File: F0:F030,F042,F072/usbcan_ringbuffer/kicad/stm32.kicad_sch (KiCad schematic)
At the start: 54 parts, among them J1 Screw_Terminal_01x03, J10 SDA, J11 PB0, J12 PB1, J13 PB4, J14 PB5, J15 PB2, J16 PB3, J17 GND, J18 GND, J19 +3.3V, J2 SCK, J20 +5V, J21 PA0, J22 PA1, J23 PA2, J24 PA3, J25 PB10, J26 PB11, J3 SWDetc, J4 USB_B, J5 MISO, J6 MOSI, J7 TX, J8 RX, J9 SCL, P1 Hole, P2 Hole, P3 Hole, P4 Hole, Q1 B0505S, SW1 SW_DIP_x01, U1 LM1117-3.3, U2 USBLC6-2SC6, U3 STM32F072C8Tx, U4 ISO1050DUB

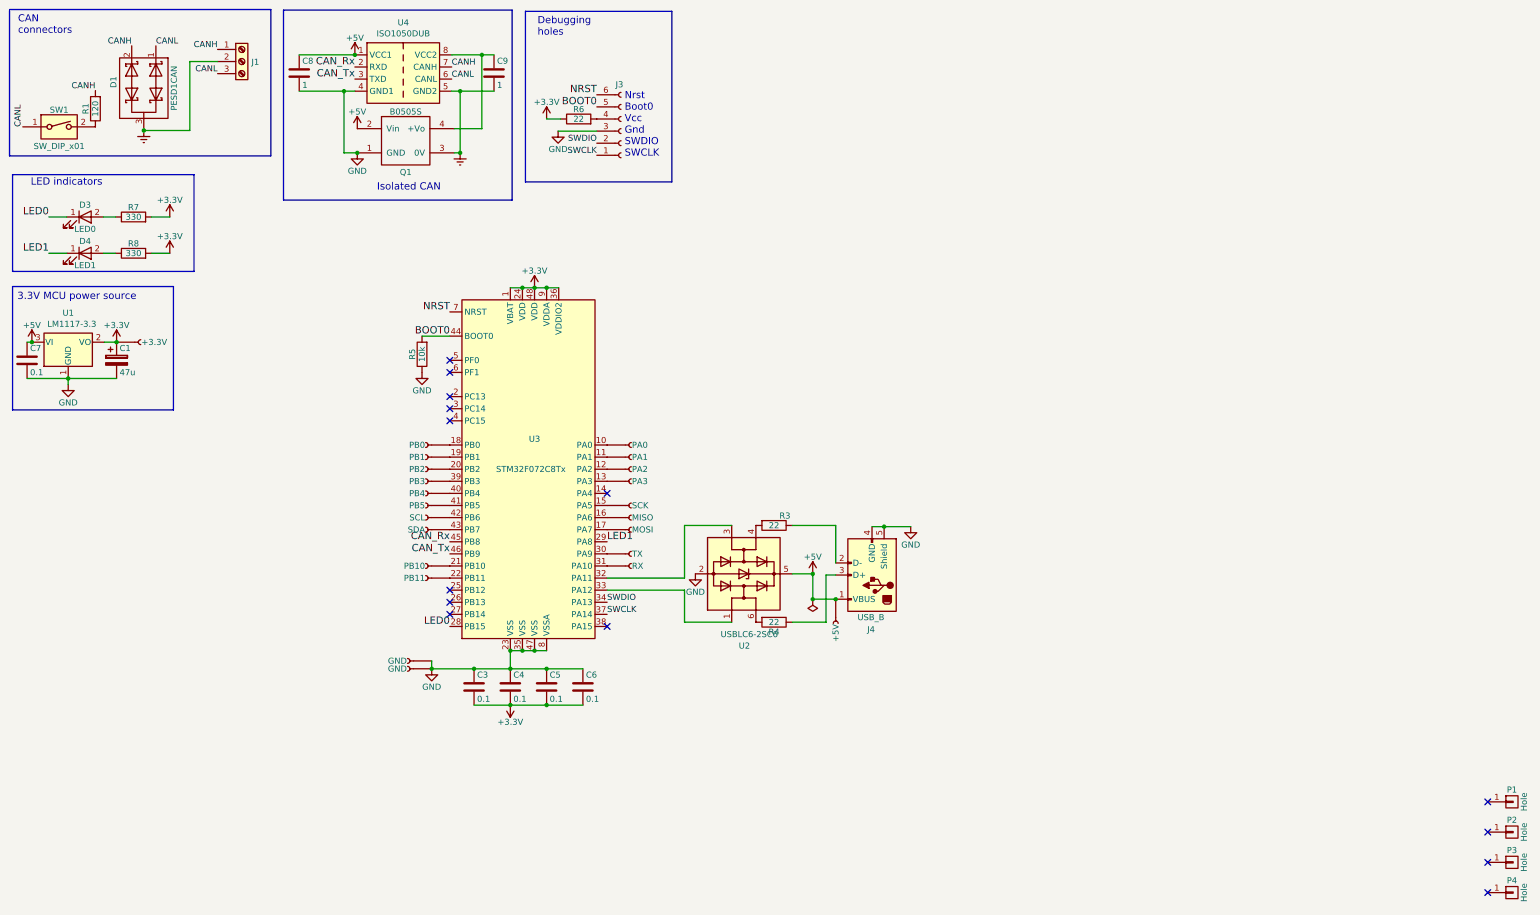
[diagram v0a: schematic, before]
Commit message: save under new kicad
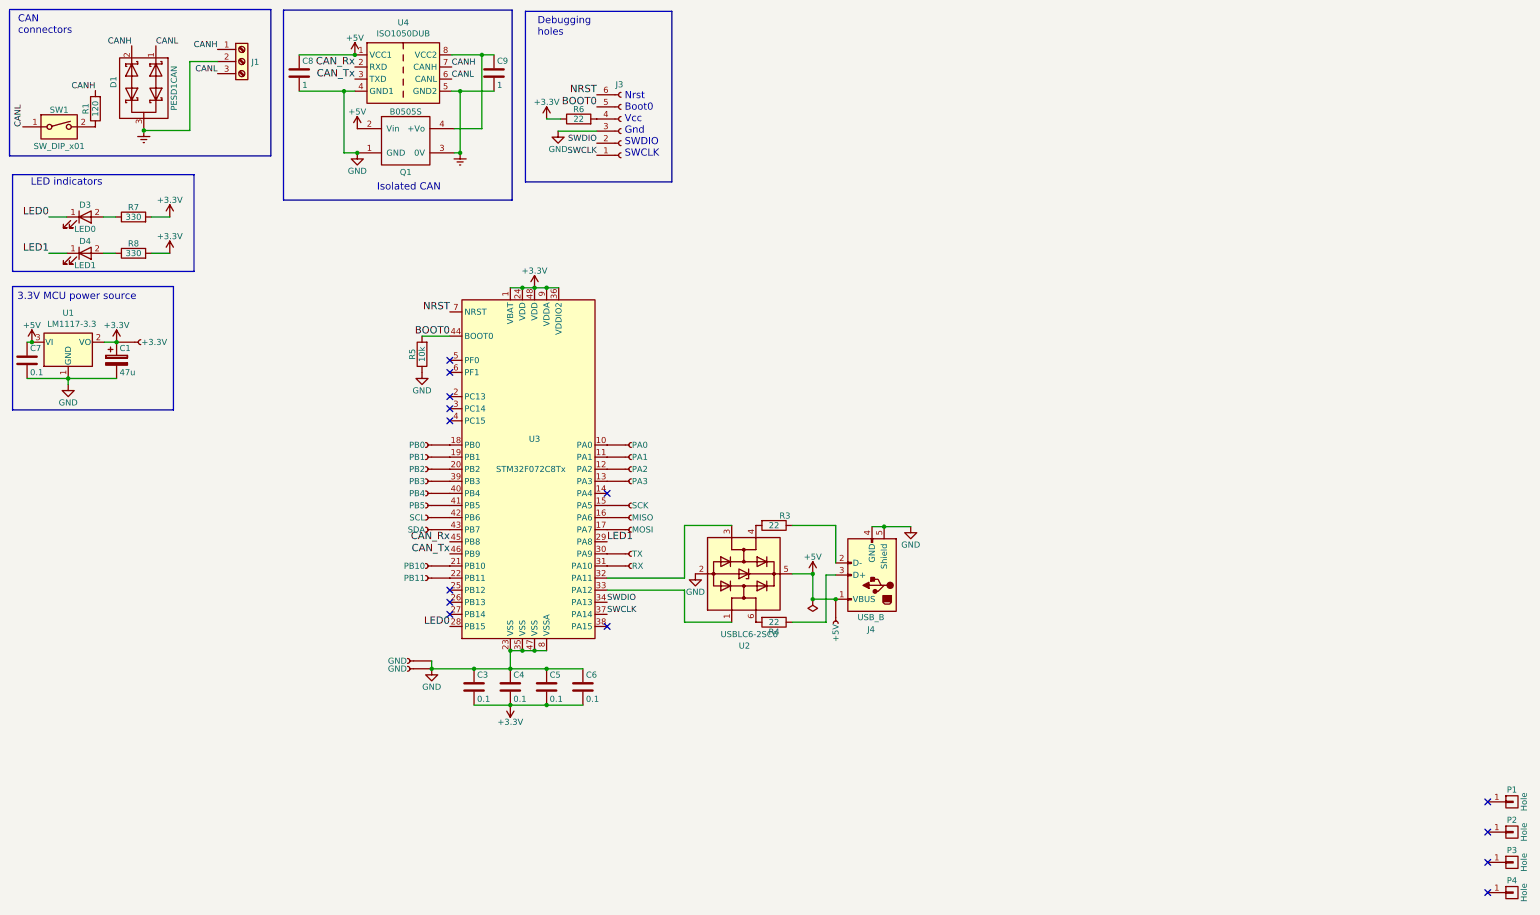
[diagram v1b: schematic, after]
